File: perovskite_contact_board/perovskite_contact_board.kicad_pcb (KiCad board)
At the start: 4 copper layers, 57 x 52.2 mm, 15 parts, among them J1 Conn_2x3, J2 Conn_2x3, J3 Conn_2x3, J4 Conn_2x3, J5 Conn2x3, J6 Conn_2x3, U1 Perovskite_CP_6_Cell, U2 Perovskite_CP_6_Cell, U3 Perovskite_CP_6_Cell, U4 MCP9808_MSOP, U5 MCP9808_MSOP, U6 MCP9808_MSOP

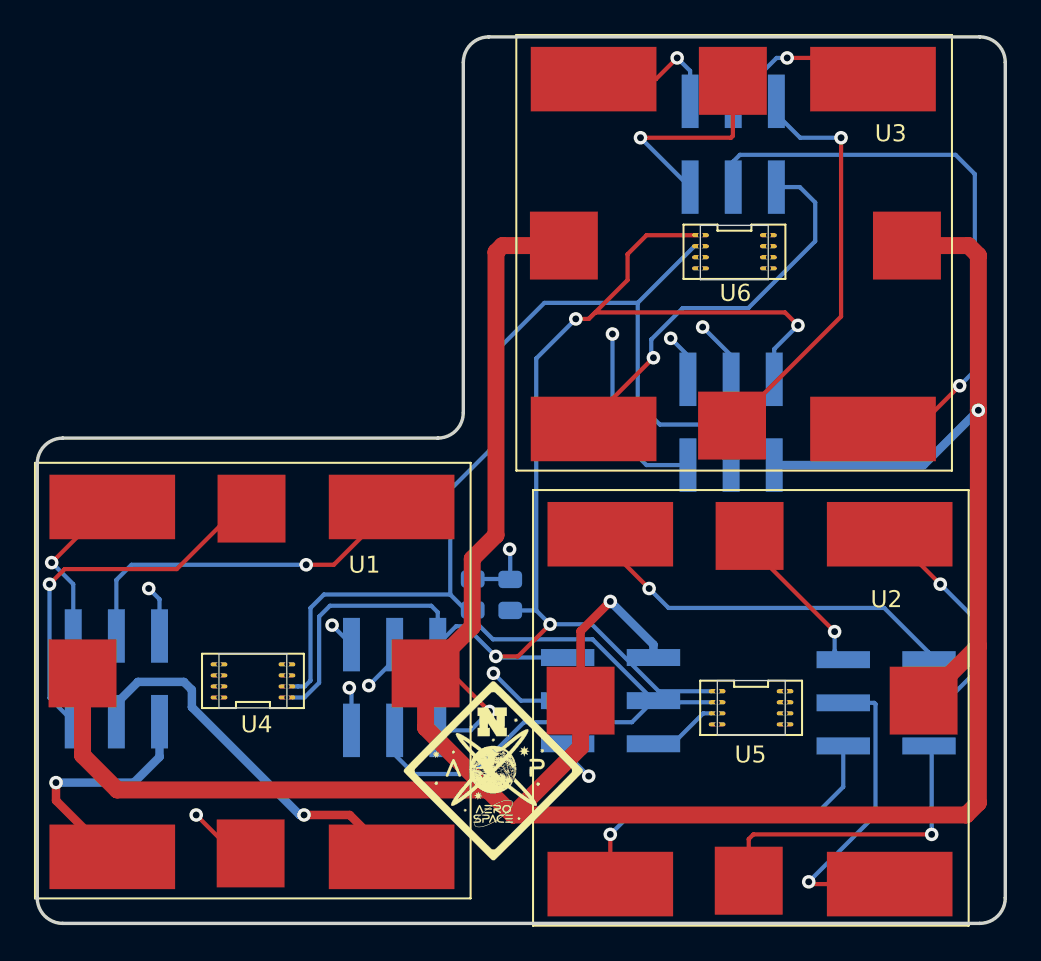
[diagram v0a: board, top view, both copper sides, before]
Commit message: pushing changes from Monday meeting
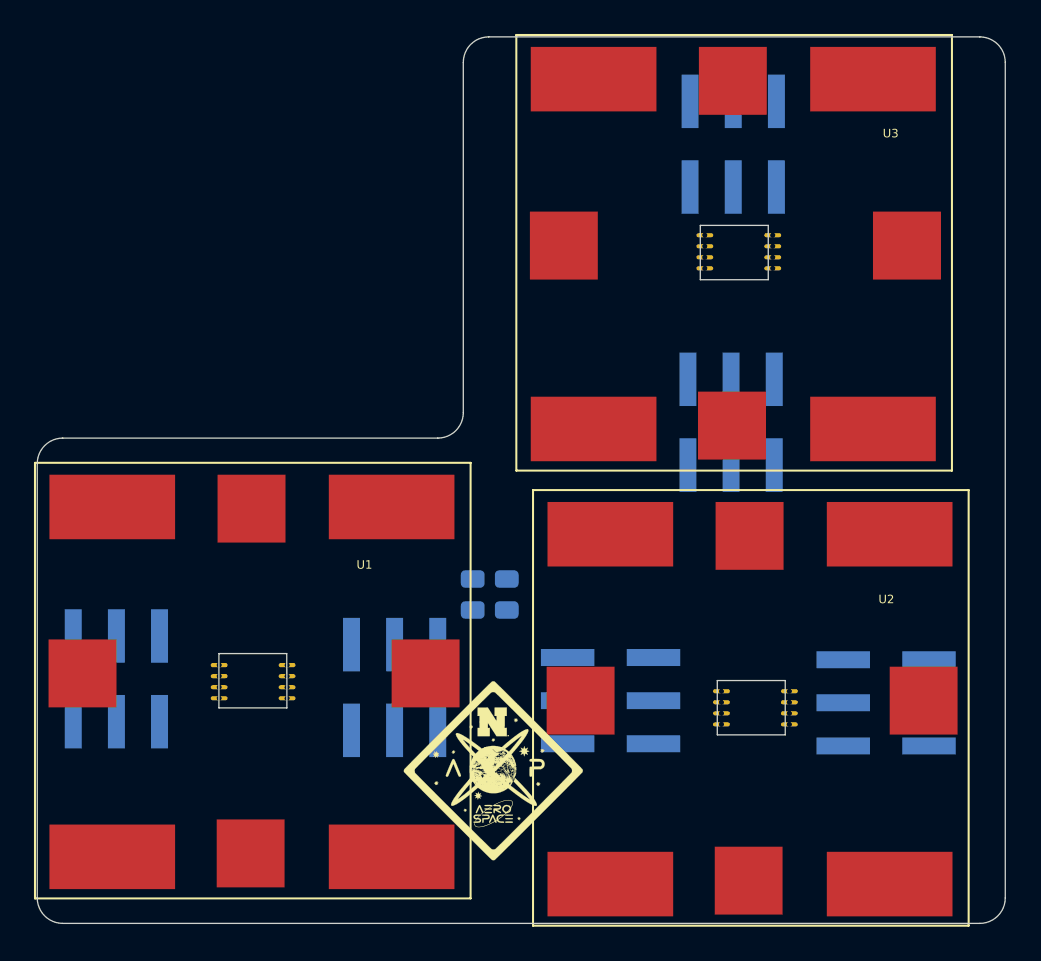
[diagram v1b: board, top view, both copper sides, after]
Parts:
- U4, U5, U6: moved to B.Cu
- moved U4 2.75 mm to (184.6, 81.7)
- moved R4 0.20 mm to (199.6, 78.0)
- turned U5 to 180 degrees
- turned U6 to 180 degrees
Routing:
- net CP: track 184.7 -> 0.00 mm, vias 3 -> 0
- net Vdd: track 116.8 -> 0.00 mm, vias 4 -> 0
- net GND: track 115.5 -> 0.00 mm, vias 3 -> 0
- net SCL: track 95.3 -> 0.30 mm
- net SDA: track 86.4 -> 0.00 mm, vias 4 -> 0
- net 16: track 35.4 -> 0.00 mm, vias 1 -> 0
- net 17: track 24.7 -> 0.00 mm, vias 1 -> 0
- net 18: track 23.8 -> 0.00 mm, vias 1 -> 0
- net 4: track 22.7 -> 0.00 mm, vias 1 -> 0
- net 7: track 22.6 -> 0.00 mm, vias 1 -> 0
- net 2: track 22.4 -> 0.00 mm, vias 1 -> 0
- net 5: track 22.2 -> 0.00 mm, vias 2 -> 0
- net 3: track 21.3 -> 0.00 mm, vias 1 -> 0
- net 12: track 20.2 -> 0.00 mm, vias 1 -> 0
- net 10: track 19.0 -> 0.00 mm, vias 1 -> 0
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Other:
- copper layers 4 -> 2
- rule trace_min: 0.2 -> 0.1524
- rule via_min_drill: 0.3 -> 0.254
- rule via_min_size: 0.4 -> 0.508
